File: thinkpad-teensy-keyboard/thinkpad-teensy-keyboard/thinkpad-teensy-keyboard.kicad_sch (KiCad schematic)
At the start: 15 parts, among them J1 2, J2 WM6787CT-ND, J3 3, Q1 220mA/50V/3.5Ω, Q2 220mA/50V/3.5Ω, U1 Teensy4.1, U2 TLV810SDBZT

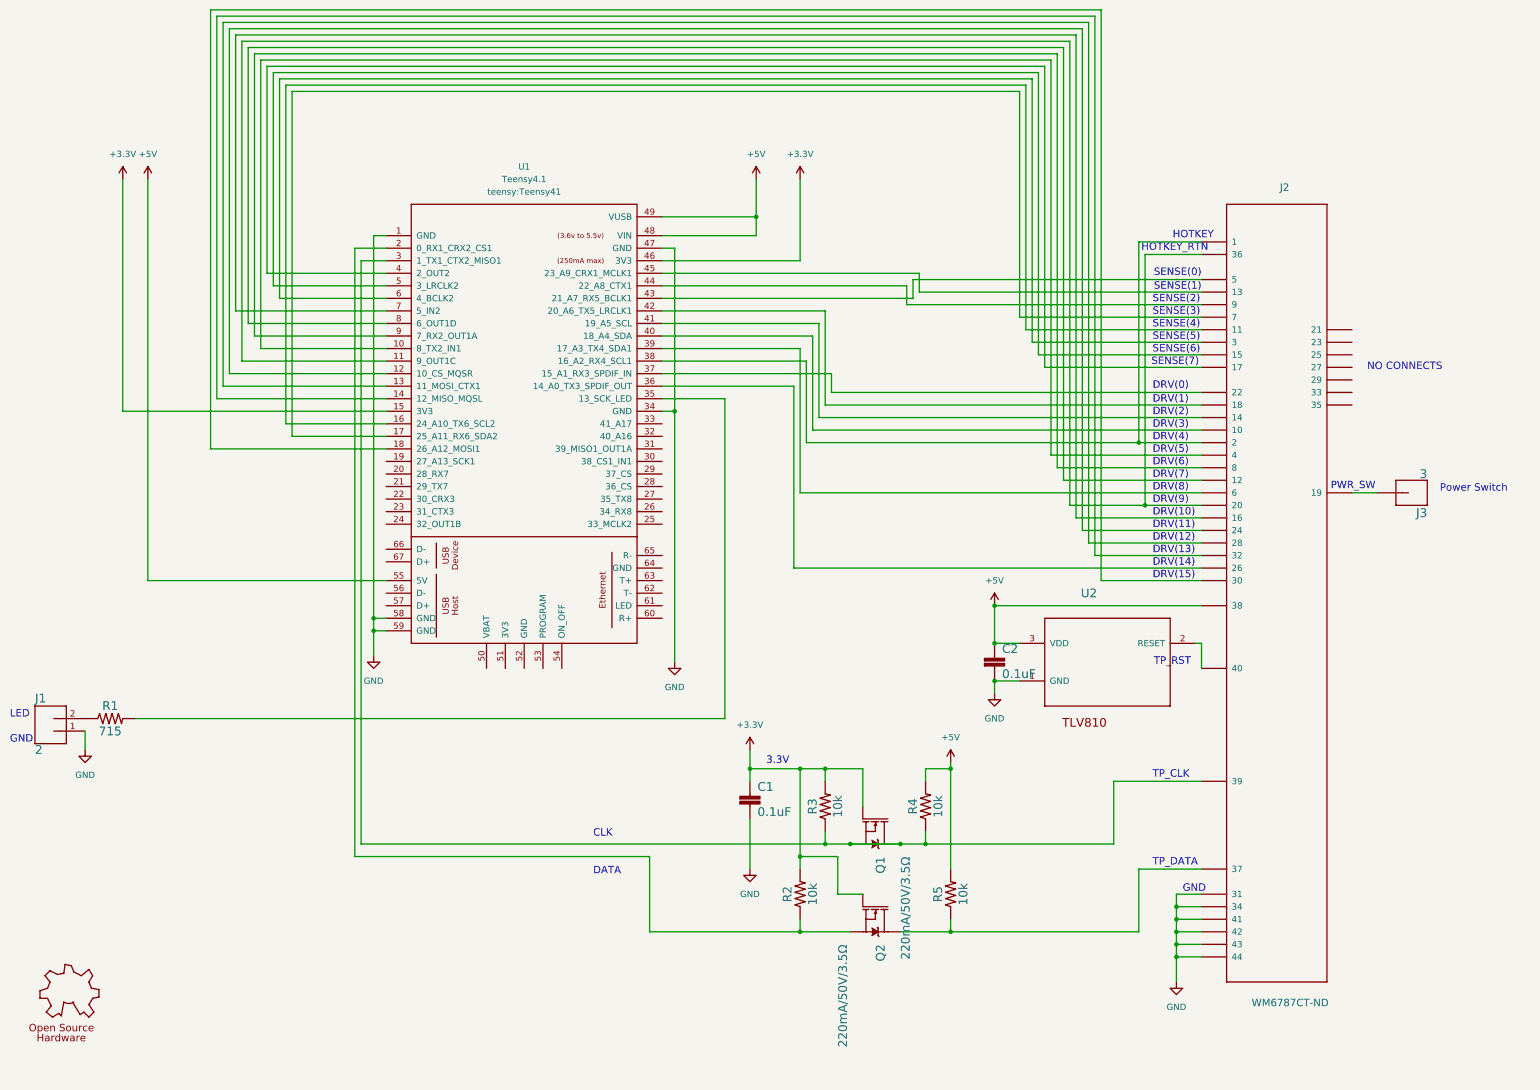
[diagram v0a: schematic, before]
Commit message: updates
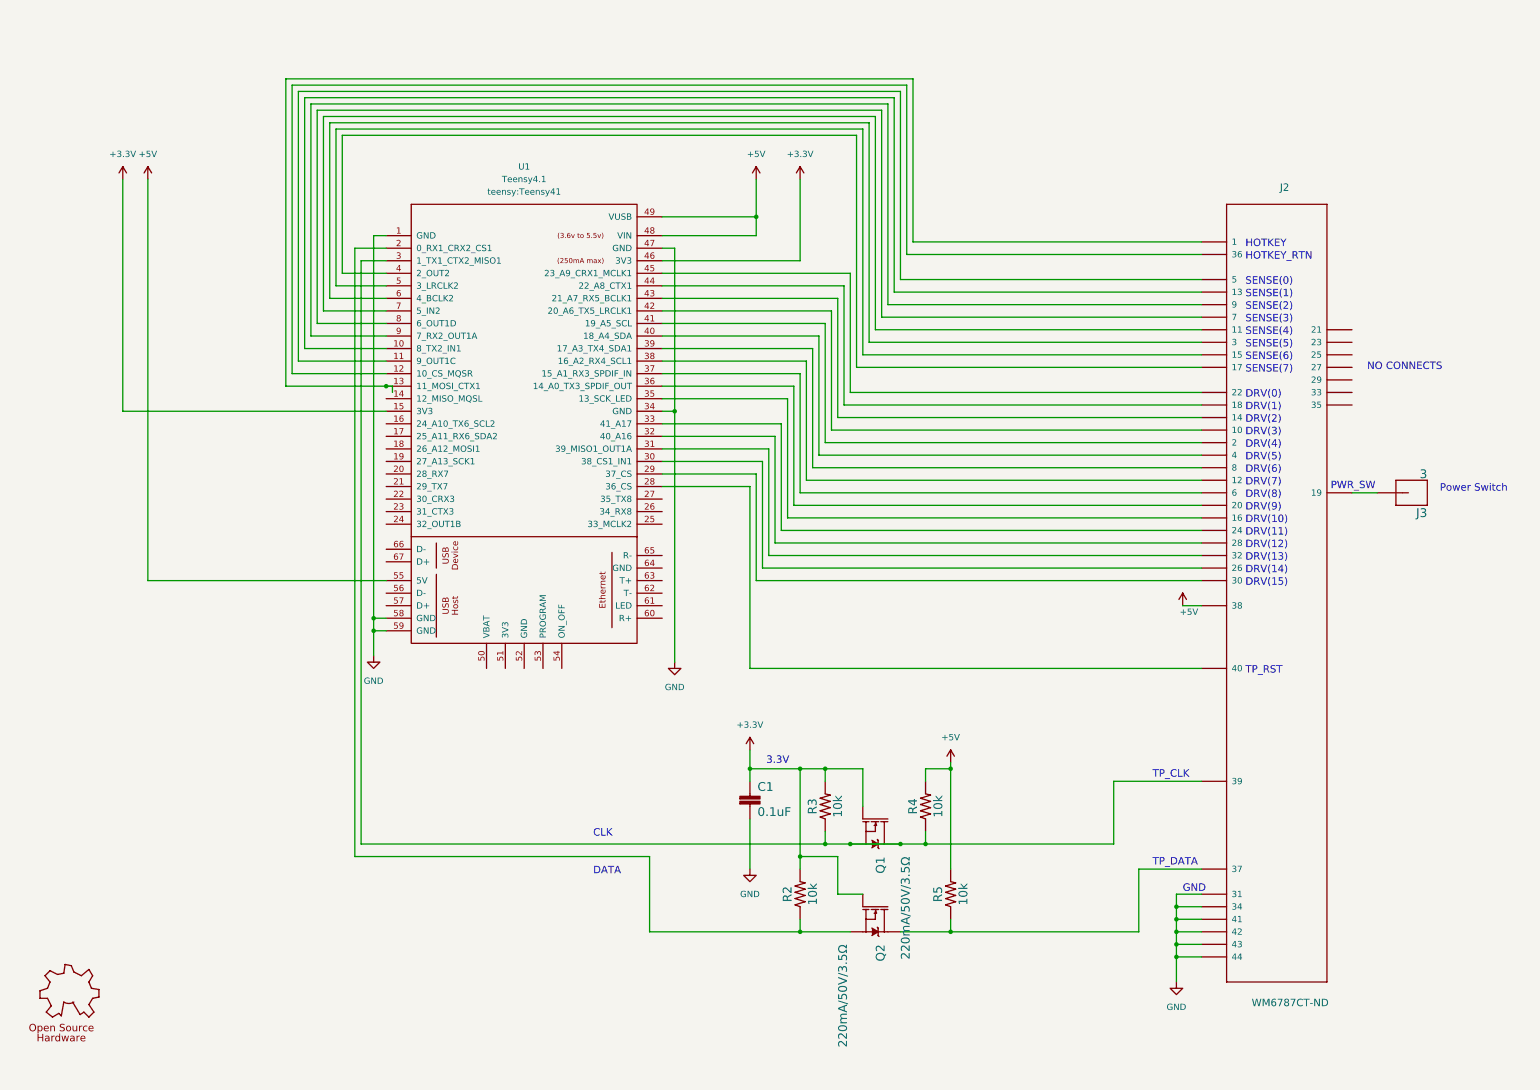
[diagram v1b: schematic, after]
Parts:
- removed C2: 0.1uF, T61_LC_Scanner:0603, symbol T61_LC_Scanner-eagle-import:0.1UF-0603-25V-(+80_-20%)
- removed J1: 2, T61_LC_Scanner:1X02, symbol T61_LC_Scanner-eagle-import:CONN_02
- removed R1: 715, T61_LC_Scanner:0603, symbol T61_LC_Scanner-eagle-import:715OHM-0603-1_10W-1%
- removed U2: TLV810SDBZT, T61_LC_Scanner:SOT95P237X112-3N, symbol T61_LC_Scanner-eagle-import:TLV810SDBZT
- C1, R2, R3, R4, R5: footprint T61_LC_Scanner:0603 -> Library:0603
- GOLD_ORB_SM1: footprint T61_LC_Scanner:OSHW_5MM -> Library:OSHW_5MM
- J2: footprint T61_LC_Scanner:WM6787CT-ND -> Library:WM6787CT-ND
- J3: footprint T61_LC_Scanner:1X01 -> Library:1X01
- Q1, Q2: footprint T61_LC_Scanner:SOT23-3 -> Library:SOT23-3
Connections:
- net at U1.10 (8_TX2_IN1): now also J2.P$13 (13); no longer J2.P$4 (4)
- net at U1.12 (10_CS_MQSR): now also J2.P$36 (36); no longer J2.P$24 (24)
- net at U1.13 (11_MOSI_CTX1): now also J2.P$1 (1); no longer J2.P$28 (28)
- net at U1.14 (12_MISO_MQSL): no longer J2.P$32 (32)
- net at U1.16 (24_A10_TX6_SCL2): no longer J2.P$11 (11)
- net at U1.17 (25_A11_RX6_SDA2): no longer J2.P$7 (7)
- net at U1.18 (26_A12_MOSI1): no longer J2.P$30 (30)
- net at U1.28 (36_CS): now also J2.P$40 (40)
- net at U1.29 (37_CS): now also J2.P$30 (30)
- net at U1.30 (38_CS1_IN1): now also J2.P$26 (26)
- net at U1.31 (39_MISO1_OUT1A): now also J2.P$32 (32)
- net at U1.32 (40_A16): now also J2.P$28 (28)
- net at U1.33 (41_A17): now also J2.P$24 (24)
- net at U1.35 (13_SCK_LED): now also J2.P$16 (16)
- net at U1.36 (14_A0_TX3_SPDIF_OUT): now also J2.P$20 (20); no longer J2.P$26 (26)
- net at U1.37 (15_A1_RX3_SPDIF_IN): now also J2.P$6 (6); no longer J2.P$22 (22)
- net at U1.39 (17_A3_TX4_SDA1): now also J2.P$8 (8); no longer J2.P$6 (6)
- net at U1.40 (18_A4_SDA): now also J2.P$4 (4); no longer J2.P$10 (10)
- net at U1.41 (19_A5_SCL): now also J2.P$2 (2); no longer J2.P$14 (14)
- net at U1.42 (20_A6_TX5_LRCLK1): now also J2.P$10 (10); no longer J2.P$18 (18)
- net at J2.P$5 (5): now also U1.11 (9_OUT1C); no longer U1.43 (21_A7_RX5_BCLK1)
- net at U1.44 (22_A8_CTX1): now also J2.P$18 (18); no longer J2.P$9 (9)
- net at U1.45 (23_A9_CRX1_MCLK1): now also J2.P$22 (22); no longer J2.P$13 (13)
- net at U1.7 (5_IN2): now also J2.P$11 (11); no longer J2.P$16 (16)
- net at J2.P$12 (12): now also U1.38 (16_A2_RX4_SCL1); no longer U1.8 (6_OUT1D)
- net at U1.9 (7_RX2_OUT1A): now also J2.P$9 (9); no longer J2.P$8 (8)
- new net: J2.P$14 (14), U1.43 (21_A7_RX5_BCLK1)
- new net: J2.P$7 (7), U1.8 (6_OUT1D)
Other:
- note removed: "LED"

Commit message: Generated Gerbers
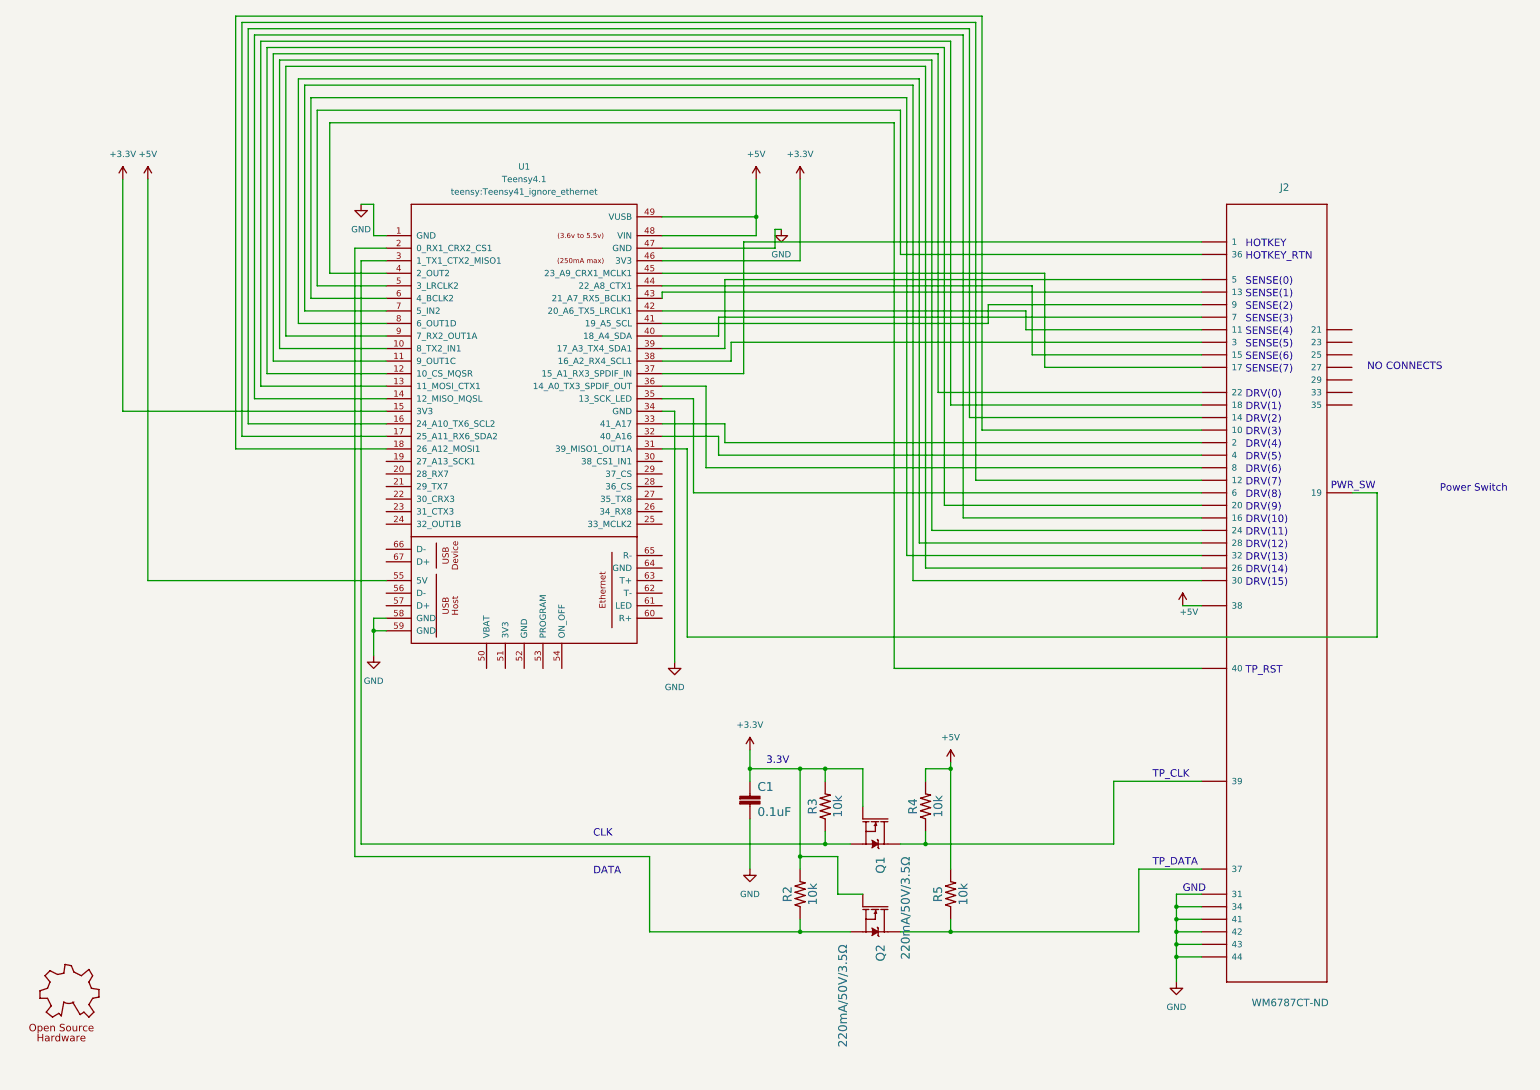
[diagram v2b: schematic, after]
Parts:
- removed J3: 3, Library:1X01, symbol T61_LC_Scanner-eagle-import:CONN_01
- U1: footprint teensy:Teensy41 -> teensy:Teensy41_ignore_ethernet
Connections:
- net at Q1.2 (S), R3.1, U1.3 (1_TX1_CTX2_MISO1): no longer J2.P$39 (39), Q1.3 (D), R4.1
- net at U1.10 (8_TX2_IN1): now also J2.P$24 (24); no longer J2.P$13 (13)
- net at U1.11 (9_OUT1C): now also J2.P$22 (22); no longer J2.P$5 (5)
- net at U1.12 (10_CS_MQSR): now also J2.P$20 (20); no longer J2.P$36 (36)
- net at U1.13 (11_MOSI_CTX1): now also J2.P$18 (18); no longer J2.P$1 (1)
- net at U1.14 (12_MISO_MQSL): now also J2.P$16 (16)
- net at U1.16 (24_A10_TX6_SCL2): now also J2.P$14 (14)
- net at U1.17 (25_A11_RX6_SDA2): now also J2.P$12 (12)
- net at U1.18 (26_A12_MOSI1): now also J2.P$10 (10)
- net at U1.28 (36_CS): no longer J2.P$40 (40)
- net at U1.29 (37_CS): no longer J2.P$30 (30)
- net at U1.30 (38_CS1_IN1): no longer J2.P$26 (26)
- net at U1.31 (39_MISO1_OUT1A): now also J2.P$19 (19); no longer J2.P$32 (32)
- net at U1.32 (40_A16): now also J2.P$4 (4); no longer J2.P$28 (28)
- net at U1.33 (41_A17): now also J2.P$2 (2); no longer J2.P$24 (24)
- net at U1.35 (13_SCK_LED): now also J2.P$6 (6); no longer J2.P$16 (16)
- net at U1.36 (14_A0_TX3_SPDIF_OUT): now also J2.P$8 (8); no longer J2.P$20 (20)
- net at U1.37 (15_A1_RX3_SPDIF_IN): now also J2.P$1 (1); no longer J2.P$6 (6)
- net at U1.38 (16_A2_RX4_SCL1): now also J2.P$3 (3); no longer J2.P$12 (12)
- net at U1.39 (17_A3_TX4_SDA1): now also J2.P$5 (5); no longer J2.P$8 (8)
- net at U1.4 (2_OUT2): now also J2.P$40 (40); no longer J2.P$17 (17)
- net at U1.40 (18_A4_SDA): now also J2.P$7 (7); no longer J2.P$4 (4)
- net at U1.41 (19_A5_SCL): now also J2.P$9 (9); no longer J2.P$2 (2)
- net at U1.42 (20_A6_TX5_LRCLK1): now also J2.P$11 (11); no longer J2.P$10 (10)
- net at U1.43 (21_A7_RX5_BCLK1): now also J2.P$13 (13); no longer J2.P$14 (14)
- net at U1.44 (22_A8_CTX1): now also J2.P$15 (15); no longer J2.P$18 (18)
- net at U1.45 (23_A9_CRX1_MCLK1): now also J2.P$17 (17); no longer J2.P$22 (22)
- net at U1.5 (3_LRCLK2): now also J2.P$36 (36); no longer J2.P$15 (15)
- net at U1.6 (4_BCLK2): now also J2.P$32 (32); no longer J2.P$3 (3)
- net at U1.7 (5_IN2): now also J2.P$30 (30); no longer J2.P$11 (11)
- net at U1.8 (6_OUT1D): now also J2.P$28 (28); no longer J2.P$7 (7)
- net at U1.9 (7_RX2_OUT1A): now also J2.P$26 (26); no longer J2.P$9 (9)
- new net: J2.P$39 (39), Q1.3 (D), R4.1
